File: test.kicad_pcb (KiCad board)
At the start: 4 copper layers, 100 x 50 mm, 110 parts, among them IC1 USBLC6-2SC6, IC2 AD9288BSTZ-40, IC3 MAX17048G+T10, IC4 BQ24074RGTR, IC5 TCA9534APWR, IC6 MCP6S91-E_MS, IC7 MCP6S91-E_MS, IC8 MCP4726A0T-E_CH, J1 PWM, K1 AQY210EHAX, K2 AQY210EHAX, Q1 SS8050-G, Q2 SS8050-G, SW1 Reset, SW2 Button, SW3 SW_DPDT_x2, U1 USB-TYPE-C-018, U10 MCP6022T-I_SN, U2 CP2102N-A02-GQFN28, U3 ESP32-WROOM-E, U4 1043, U5 1043, U6 LD1086DT33TR, U7 LD1086DT33TR, U8 MCP6022T-I_SN, U9 MCP6022T-I_SN

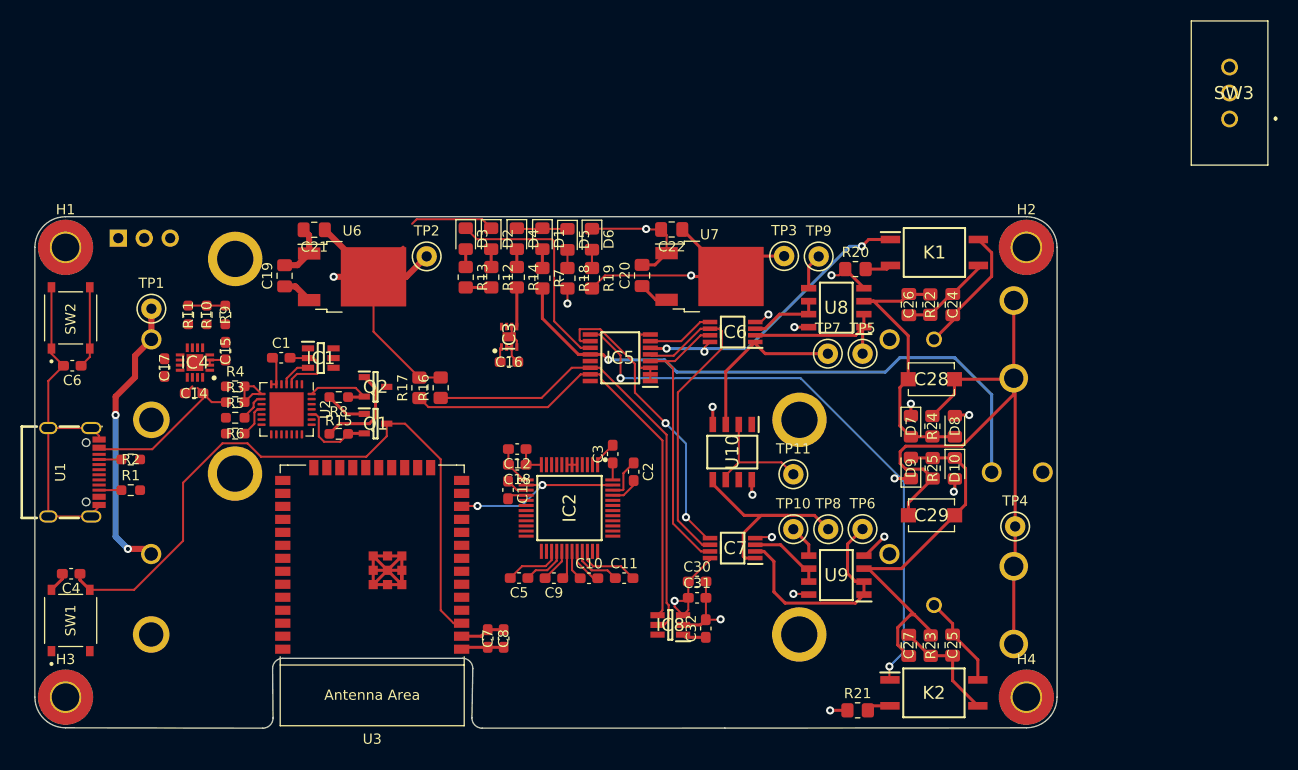
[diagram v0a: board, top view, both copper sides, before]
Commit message: routing
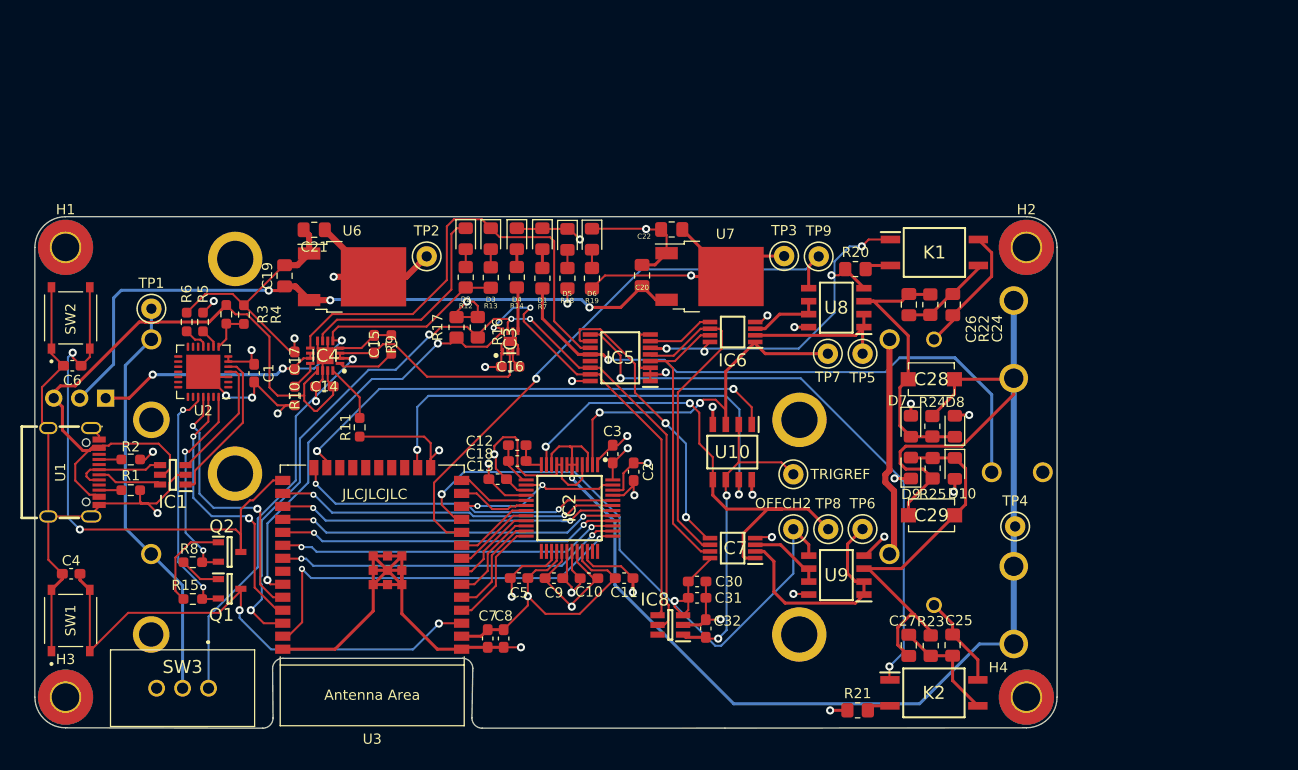
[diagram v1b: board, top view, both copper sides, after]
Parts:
- moved SW3 118.0 mm to (114.5, 94.7), turned to 90 degrees
- moved Q1 21.6 mm to (119.0, 85.4)
- moved R15 21.6 mm to (115.5, 86.4)
- moved Q2 21.6 mm to (119.0, 81.8)
- moved R8 21.6 mm to (115.5, 82.8)
- moved R11 20.1 mm to (131.8, 69.6), turned to -90 degrees
- moved IC1 18.4 mm to (113.5, 74.2), turned to 180 degrees
- moved R9 16.5 mm to (134.9, 61.5)
- moved JP1 15.7 mm to (106.9, 66.8), turned to 90 degrees
- moved C15 14.6 mm to (133.2, 61.5)
- moved IC4 12.8 mm to (128.4, 62.6)
- moved C14 12.8 mm to (128.3, 65.6)
- moved C17 12.8 mm to (125.4, 63.1)
- moved R6 11.9 mm to (114.8, 59.3), turned to 90 degrees
- moved R10 11.7 mm to (125.4, 66.5), turned to -90 degrees
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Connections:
- C10 pad 2: GNDA -> GND
- C20 pad 2: GNDA -> GND
- C22 pad 2: GNDA -> GND
- C3 pad 2: GNDA -> GND
- C30 pad 2: GNDA -> GND
- C31 pad 2: GNDA -> GND
- C32 pad 2: GNDA -> GND
- C9 pad 2: GNDA -> GND
- D10 pad 2: GNDA -> GND
- D6 pad 1: GNDA -> GND
- D8 pad 2: GNDA -> GND
- IC2 pad 1: GNDA -> GND
- IC2 pad 10: GNDA -> GNDREF
- IC2 pad 29: GNDA -> GND
- IC2 pad 3: GNDA -> GNDREF
- IC2 pad 32: GNDA -> GND
- IC6 pad 4: GNDA -> GND
- IC7 pad 4: GNDA -> GND
- IC8 pad 2: GNDA -> GND
- R20 pad 1: GNDA -> GND
- R21 pad 1: GNDA -> GND
- U10 pad 4: GNDA -> GND
- U3 pad 13: /CH1_D6 -> /CH2_D6
- U3 pad 14: /CH1_D7 -> /CH2_D7
- U3 pad 24: /CH2_D0 -> /CH1_D7
- U3 pad 26: /CH2_D1 -> /CH1_D6
- U3 pad 27: /CH2_D3 -> /CH1_D5
- U3 pad 28: /CH2_D4 -> /CH1_D4
- U3 pad 29: /CH2_D2 -> /CH1_D3
- U3 pad 30: /CH2_D5 -> /CH1_D2
- U3 pad 31: /CH2_D6 -> /CH1_D1
- U3 pad 37: /CH2_D7 -> /CH1_D0
- U3 pad 4: /CH1_D0 -> /CH2_D0
- U3 pad 5: /CH1_D1 -> /CH2_D1
- U3 pad 6: /CH1_D2 -> /CH2_D2
- U3 pad 7: /CH1_D3 -> /CH2_D3
- U3 pad 8: /CH1_D4 -> /CH2_D4
- U3 pad 9: /CH1_D5 -> /CH2_D5
- U7 pad 1: GNDA -> GND
- U8 pad 4: GNDA -> GND
- U9 pad 4: GNDA -> GND
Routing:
- net GND: track 114.2 -> 320.4 mm, vias 0 -> 28
- net GNDREF: track 69.6 -> 137.4 mm, vias 0 -> 1
- net Net-(C19-Pad1): track 5.91 -> 68.1 mm, vias 0 -> 3
- net Net-(C15-Pad1): track 4.26 -> 64.2 mm, vias 0 -> 1
- net +5V: track 16.2 -> 71.5 mm
- net Offset_CH2: track 3.21 -> 58.3 mm, vias 0 -> 1
- net Offset_CH1: track 3.51 -> 57.5 mm, vias 0 -> 1
- net Trigger_CH1: track 0.00 -> 49.5 mm, vias 0 -> 2
- net Trigger_CH2: track 0.00 -> 48.3 mm, vias 0 -> 2
- net +3V3: track 101.9 -> 148.9 mm, vias 2 -> 9
- net IO0: track 8.03 -> 54.7 mm, vias 0 -> 2
- net Net-(C17-Pad1): track 2.50 -> 48.3 mm, vias 0 -> 3
- net GNDA: track 45.7 -> 0.00 mm, vias 10 -> 0
- net SCL_I2C: track 45.6 -> 89.9 mm, vias 0 -> 4
- net /CH1_D0: track 0.00 -> 40.2 mm, vias 0 -> 2
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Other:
- board text added: "JLCJLCJLC"
